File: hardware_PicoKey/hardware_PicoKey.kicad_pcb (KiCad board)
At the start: 2 copper layers, 36.9 x 18.5 mm, 36 parts, among them J1 USB_A, SW1 SW_Push, SW2 SW_Push, U1 RP2350A-QFN60, U2 AMS1117S-3.3, U3 W25Q128JVS, Y1 Crystal_GND24

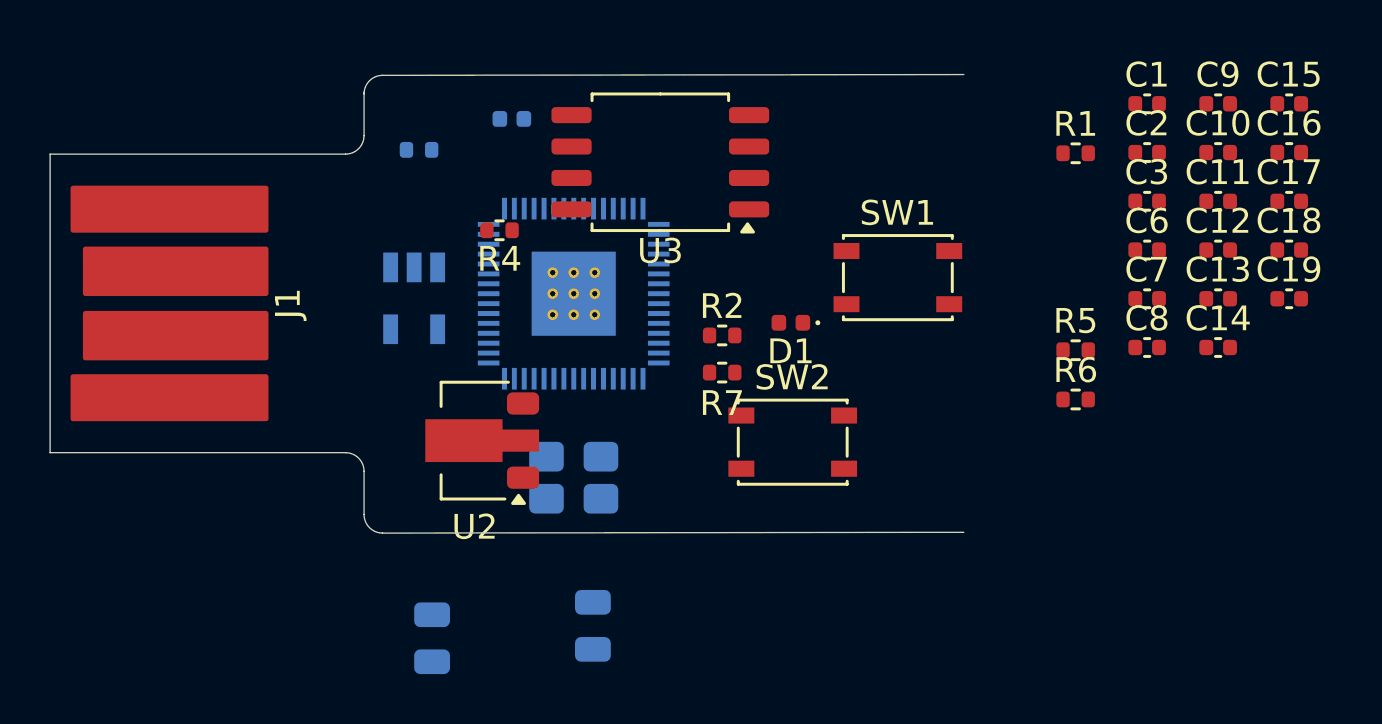
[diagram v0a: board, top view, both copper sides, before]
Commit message: pcb
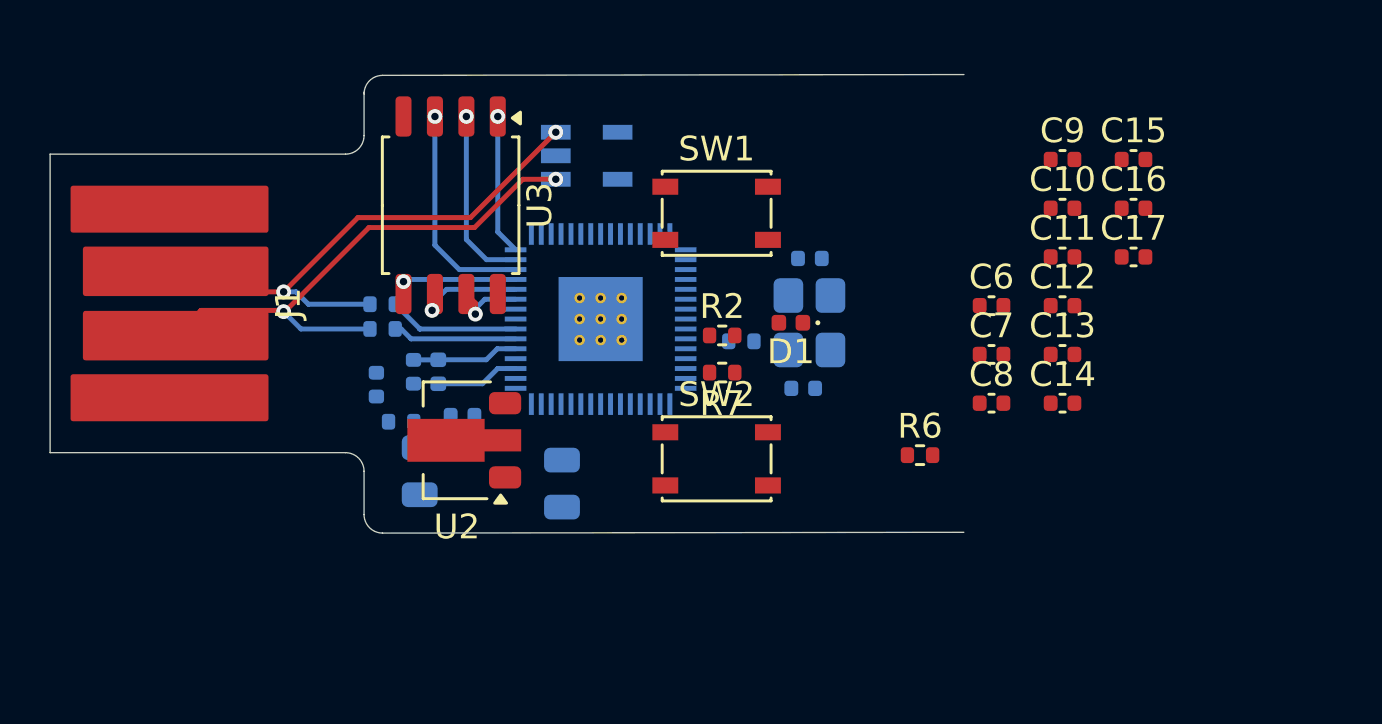
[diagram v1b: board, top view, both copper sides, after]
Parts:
- C1, C18, C19, C2, C3, R1, R4, R5: moved to B.Cu
- moved C2 32.5 mm to (136.2, 71.8), turned to 90 degrees
- moved C3 30.4 mm to (137.8, 71.2), turned to -90 degrees
- moved C1 30.4 mm to (139.7, 73.0)
- moved R1 29.3 mm to (137.2, 73.2)
- moved C18 20.4 mm to (153.5, 71.9)
- moved C19 19.4 mm to (153.8, 66.7), turned to 180 degrees
- moved R5 13.5 mm to (151.0, 70.0), turned to 180 degrees
- moved Y1 11.4 mm to (153.8, 69.2), turned to -90 degrees
- moved L1 10.6 mm to (138.8, 71.2), turned to 90 degrees
- moved D2 9.05 mm to (144.8, 62.5), turned to 0 degrees
- moved U3 8.65 mm to (139.2, 64.5), turned to -90 degrees
- moved SW1 7.77 mm to (150.0, 64.8)
- moved C4 6.77 mm to (138.0, 75.2), turned to -90 degrees
- moved C10 6.68 mm to (164.0, 64.6)
- moved C11 6.68 mm to (164.0, 66.6)
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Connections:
- D2 pad 1: USB_DP -> USB_DM
- D2 pad 2: unconnected-(D2-GND-Pad2) -> GND
- D2 pad 3: USB_DM -> USB_DP
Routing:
- net USB_DP: track 0.00 -> 22.1 mm, vias 0 -> 2
- net USB_DM: track 0.00 -> 21.9 mm, vias 0 -> 2
- net QSPI_SD2: track 0.00 -> 8.87 mm, vias 0 -> 1
- net QSPI_SD1: track 0.00 -> 7.30 mm, vias 0 -> 1
- net QSPI_SS: track 0.00 -> 5.69 mm, vias 0 -> 1
- net Net-(U1-USB_DP): track 0.00 -> 5.28 mm
- net QSPI_SD0: track 0.00 -> 5.07 mm, vias 0 -> 1
- net Net-(U1-USB_DM): track 0.00 -> 5.03 mm
- net QSPI_SCLK: track 0.00 -> 4.59 mm, vias 0 -> 1
- net 1v1: track 0.00 -> 4.32 mm
- net Net-(U1-VREG_LX): track 0.00 -> 3.38 mm
- net QSPI_SD3: track 0.00 -> 2.97 mm, vias 0 -> 1
